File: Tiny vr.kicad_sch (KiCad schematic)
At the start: 0 parts

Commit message: second commit because no data was in the first file
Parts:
- added C1, C2: 10uf, symbol Device:C
- added D1, D2: LED, Package_TO_SOT_SMD:TSOT-23-6, symbol Device:LED
- added J1: USB_C_Receptacle_USB2.0_14P, Package_DFN_QFN:WDFN-10-1EP_3x3mm_P0.5mm_EP1.8x2.5mm, symbol Connector:USB_C_Receptacle_USB2.0_14P
- added R1, R2: 10k, Package_DIP:DIP-8_W7.62mm, symbol Device:R
- added R3, R4: 5.1k, Package_DIP:DIP-8_W7.62mm, symbol Device:R
- added U1: ESP32-S3-MINI-1, RF_Module:ESP32-S2-MINI-1, symbol RF_Module:ESP32-S3-MINI-1
- added U2: LD1117S33TR_SOT223, Package_TO_SOT_SMD:SOT-223-3_TabPin2, symbol Regulator_Linear:LD1117S33TR_SOT223
- added U3: TP4057, Package_TO_SOT_SMD:TSOT-23-6, symbol Battery_Management:TP4057
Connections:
- new net: R2.1, U3.6 (PROG)
- new net: C1.1, J1.A4 (VBUS), J1.A9 (VBUS), J1.B4 (VBUS), J1.B9 (VBUS), R1.1, U3.4 (V_{CC})
- new net: D1.2 (A), D2.2 (A), R1.2
- new net: J1.A5 (CC1), R4.1
- new net: J1.A6 (D+), U1.24 (USB_D+)
- new net: J1.A7 (D-), U1.23 (USB_D-)
- new net: J1.B5 (CC2), R3.1
- new net: D2.1 (K), U3.5 (STDBY)
- new net: D1.1 (K), U3.1 (~{CHRG})
- new net: U1.3 (3V3), U2.2 (VO)
- new net +BATT: C2.1, U2.3 (VI), U3.3 (BAT)
- new net -BATT: C1.2, C2.2, J1.A1 (GND), J1.A12 (GND), J1.B1 (GND), J1.B12 (GND), J1.SH (SHIELD), R2.2, R3.2, R4.2, U1.1 (GND), U1.2 (GND), U1.42 (GND), U1.43 (GND), U1.46 (GND), U1.47 (GND), U1.48 (GND), U1.49 (GND), U1.50 (GND), U1.51 (GND), U1.52 (GND), U1.53 (GND), U1.54 (GND), U1.55 (GND), U1.56 (GND), U1.57 (GND), U1.58 (GND), U1.59 (GND), U1.60 (GND), U1.61 (GND), U1.62 (GND), U1.63 (GND), U1.64 (GND), U1.65 (GND), U2.1 (GND), U3.2 (GND)

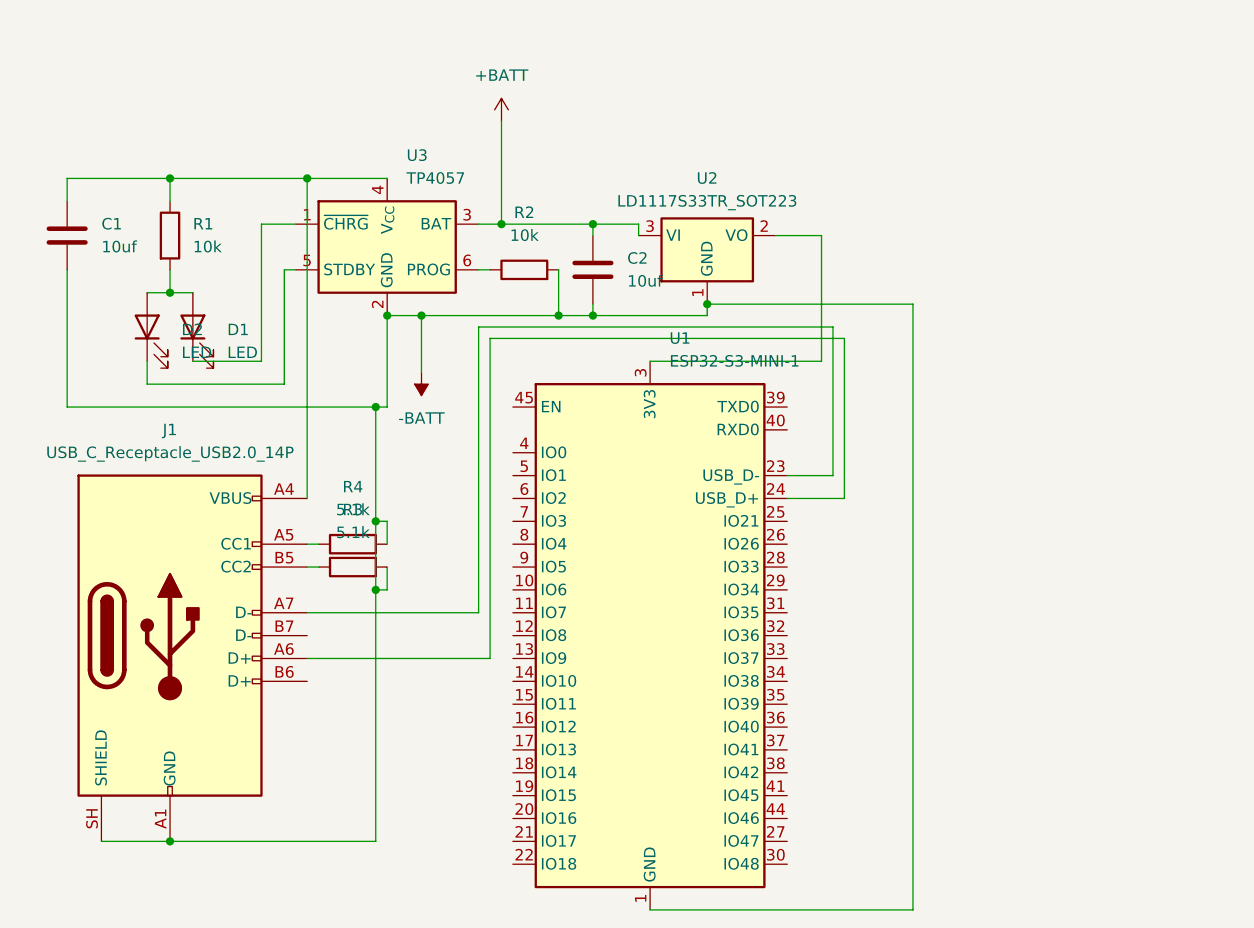
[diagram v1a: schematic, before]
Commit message: updated finished routing
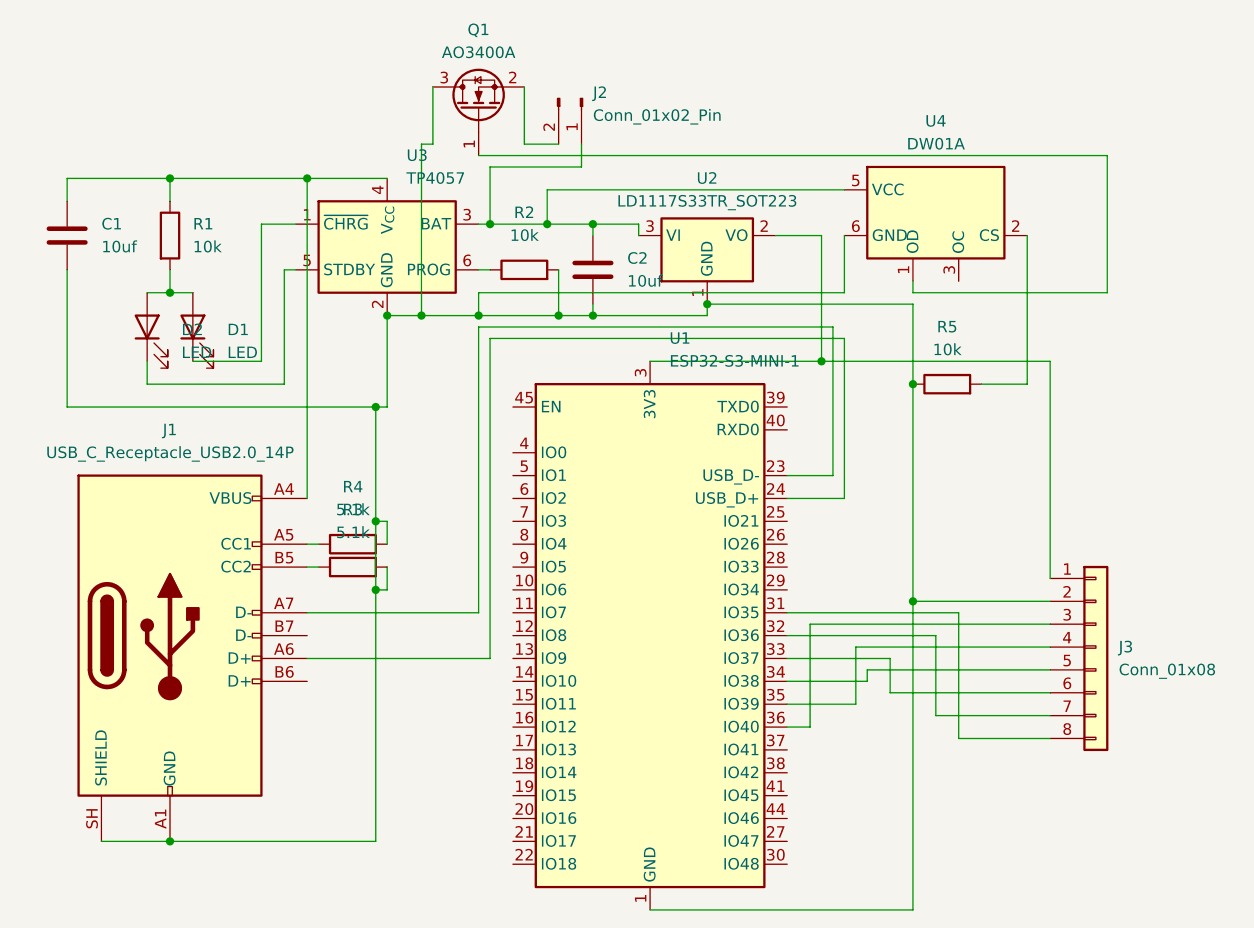
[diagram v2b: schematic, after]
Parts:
- added J2: Conn_01x02_Pin, Connector_PinHeader_2.54mm:PinHeader_1x02_P2.54mm_Horizontal, symbol Connector:Conn_01x02_Pin
- added J3: Conn_01x08, Connector_PinHeader_2.54mm:PinHeader_1x08_P2.54mm_Horizontal, symbol Connector_Generic:Conn_01x08
- added Q1: AO3400A, Package_TO_SOT_SMD:SOT-23, symbol Transistor_FET:AO3400A
- added R5: 10k, Resistor_SMD:R_0805_2012Metric, symbol Device:R
- added U4: DW01A, Package_TO_SOT_SMD:SOT-23-6, symbol Battery_Management:DW01A
- C1, C2: footprint (none) -> Capacitor_THT:C_Disc_D3.0mm_W2.0mm_P2.50mm
- D1, D2: footprint Package_TO_SOT_SMD:TSOT-23-6 -> LED_SMD:LED_01005_0402Metric
- J1: footprint Package_DFN_QFN:WDFN-10-1EP_3x3mm_P0.5mm_EP1.8x2.5mm -> Connector_USB:USB_C_Receptacle_GCT_USB4105-xx-A_16P_TopMnt_Horizontal
- R1, R2, R3, R4: footprint Package_DIP:DIP-8_W7.62mm -> Resistor_SMD:R_0805_2012Metric
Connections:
- net at U1.3 (3V3), U2.2 (VO): now also J3.1 (Pin_1)
- net at U1.31 (IO35): now also J3.8 (Pin_8)
- net at U1.32 (IO36): now also J3.7 (Pin_7)
- net at U1.33 (IO37): now also J3.6 (Pin_6)
- net at U1.34 (IO38): now also J3.5 (Pin_5)
- net at U1.35 (IO39): now also J3.4 (Pin_4)
- net at U1.36 (IO40): now also J3.3 (Pin_3)
- net +BATT: no longer names the net of C2.1, U2.3 (VI), U3.3 (BAT)
- net +BATT: now also J2.1 (Pin_1), U4.5 (VCC)
- net -BATT: no longer names the net of C1.2, C2.2, J1.A1 (GND), J1.A12 (GND), J1.B1 (GND), J1.B12 (GND), J1.SH (SHIELD), R2.2, R3.2, R4.2, U1.1 (GND), U1.2 (GND), U1.42 (GND), U1.43 (GND), U1.46 (GND), U1.47 (GND), U1.48 (GND), U1.49 (GND), U1.50 (GND), U1.51 (GND), U1.52 (GND), U1.53 (GND), U1.54 (GND), U1.55 (GND), U1.56 (GND), U1.57 (GND), U1.58 (GND), U1.59 (GND), U1.60 (GND), U1.61 (GND), U1.62 (GND), U1.63 (GND), U1.64 (GND), U1.65 (GND), U2.1 (GND), U3.2 (GND)
- net -BATT: now also J3.2 (Pin_2), Q1.3 (D), R5.1, U4.6 (GND)
- new net: R5.2, U4.2 (CS)
- new net: Q1.1 (G), U4.1 (OD)
- new net: J2.2 (Pin_2), Q1.2 (S)
